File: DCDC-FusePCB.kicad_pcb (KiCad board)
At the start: 2 copper layers, 59 x 39 mm, 11 parts, among them J1 Conn_01x02_Socket, J2 Conn_01x02_Socket

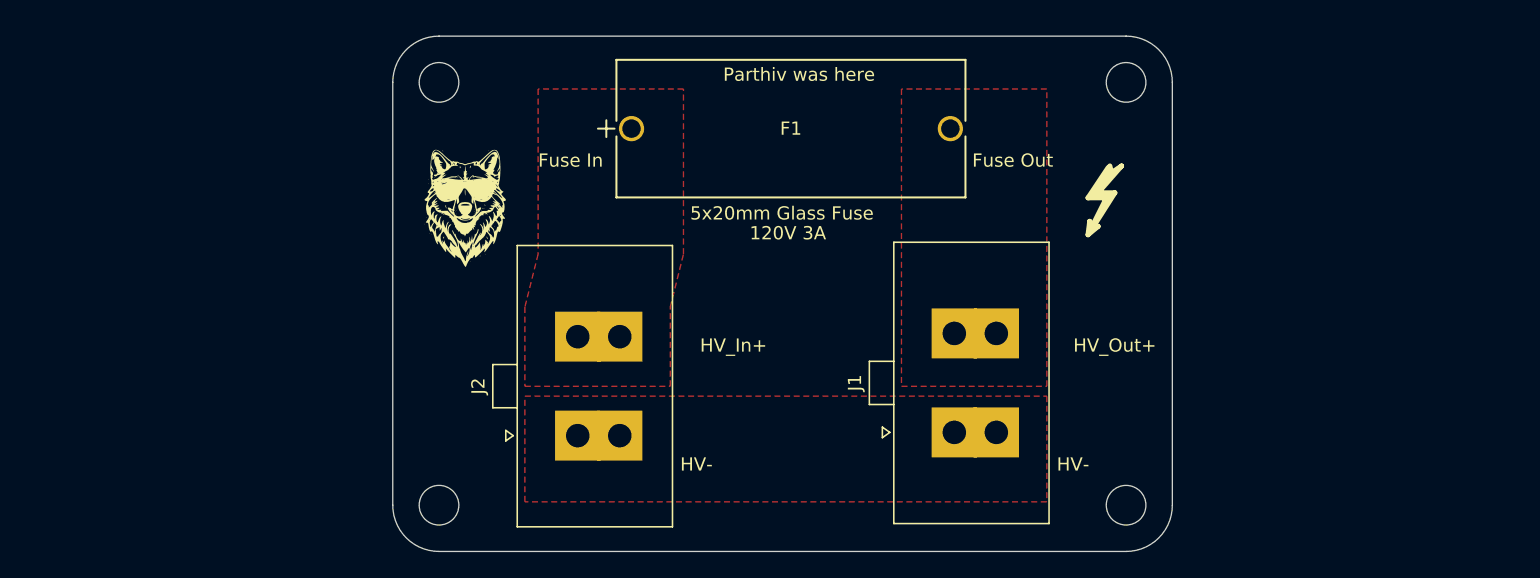
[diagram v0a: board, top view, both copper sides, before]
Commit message: precharge board
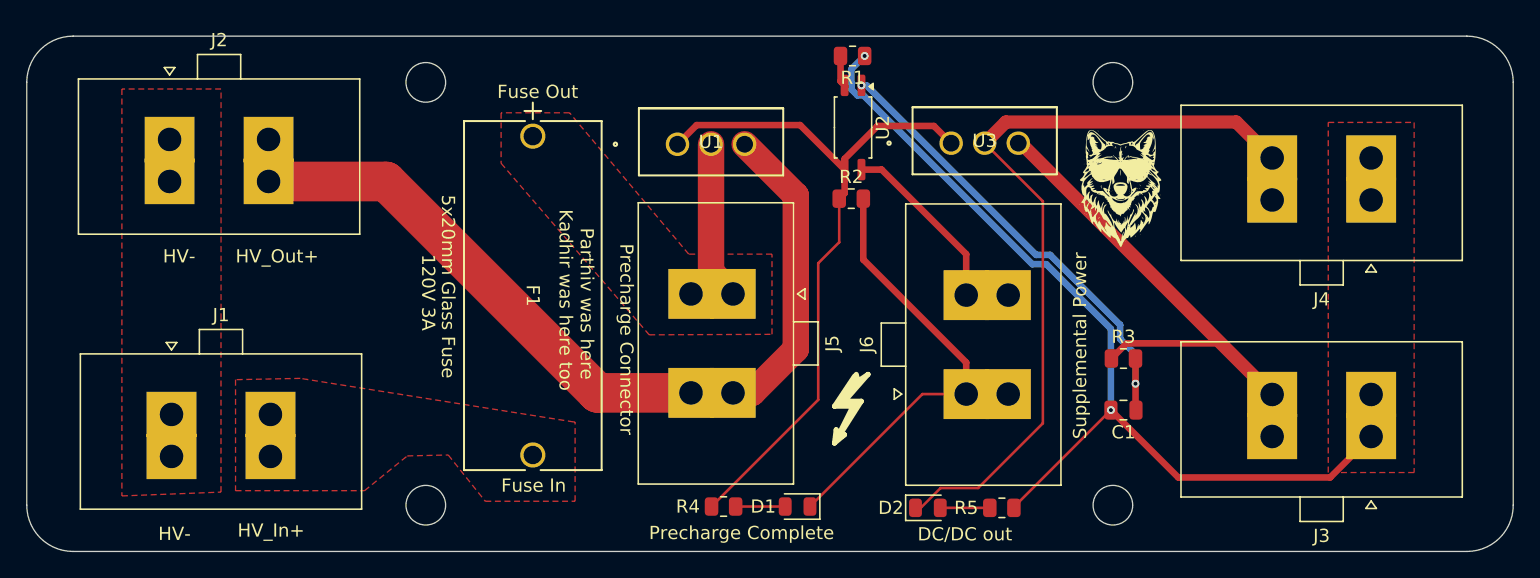
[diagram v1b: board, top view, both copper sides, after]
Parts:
- added C1: 4.7uF, Capacitor_SMD:C_0805_2012Metric, F.Cu at (164.8, 95.3)
- added D1: LED, LED_SMD:LED_0805_2012Metric, F.Cu at (140.1, 102.6)
- added D2: LED, LED_SMD:LED_0805_2012Metric, F.Cu at (150.0, 102.7)
- added J3: Conn_01x02_Socket, Connector_Molex:Molex_Sabre_43160-0102_1x02_P7.49mm_Vertical, F.Cu at (183.5, 94.1)
- added J4: Conn_01x02_Socket, Connector_Molex:Molex_Sabre_43160-0102_1x02_P7.49mm_Vertical, F.Cu at (183.5, 76.2)
- added J5: Precharge Resistor Breakout, Connector_Molex:Molex_Sabre_43160-0102_1x02_P7.49mm_Vertical, F.Cu at (132.1, 86.5)
- added J6: Conn_01x02_Socket, Connector_Molex:Molex_Sabre_43160-0102_1x02_P7.49mm_Vertical, F.Cu at (156.1, 94.1)
- added R1: 10k, Resistor_SMD:R_0805_2012Metric, F.Cu at (144.3, 68.5)
- added R2: 10k, Resistor_SMD:R_0805_2012Metric, F.Cu at (144.2, 79.3)
- added R3: 100k, Resistor_SMD:R_0805_2012Metric, F.Cu at (164.8, 91.4)
- added R4: 22.1k, Resistor_SMD:R_0805_2012Metric, F.Cu at (134.5, 102.6)
- added R5: 22.1k, Resistor_SMD:R_0805_2012Metric, F.Cu at (155.6, 102.7)
- added U1: FDP3651U, footprints:TO-220-3_16P51X10P67_ONS, F.Cu at (131.0, 75.2)
- added U2: TCMT1100, Package_SO:SOP-4_4.4x2.6mm_P1.27mm, F.Cu at (144.3, 73.9)
- added U3: FDP3651U, footprints:TO-220-3_16P51X10P67_ONS, F.Cu at (151.8, 75.1)
- moved J1 62.5 mm to (92.8, 98.8), turned to 0 degrees
- moved G*** 49.6 mm to (164.6, 78.5)
- moved J2 39.1 mm to (92.6, 78.0), turned to 0 degrees
- moved REF** 24.8 mm to (143.3, 95.8)
- moved G*** 23.4 mm to (133.1, 100.6)
- moved G*** 15.7 mm to (153.7, 96.6)
- moved F1 7.49 mm to (120.1, 74.6), turned to -90 degrees
- moved REF** 1.00 mm to (164.0, 70.5)
- moved REF** 1.00 mm to (112.0, 102.5)
- moved REF** 1.00 mm to (112.0, 70.5)
- moved REF** 1.00 mm to (164.0, 102.5)
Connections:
- net Net-(J1-Pin_1) renamed GNDin
- net Net-(J1-Pin_2) renamed HVin
- F1 pad 1: Net-(J2-Pin_2) -> Net-(J5-Pin_1)
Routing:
- net GNDout: track 0.00 -> 69.8 mm, vias 0 -> 2
- net Net-(J2-Pin_2): track 0.00 -> 61.8 mm
- net DC/DC out: track 0.00 -> 58.9 mm
- net Gate_Drive: track 0.00 -> 54.8 mm
- net LowPassIn: track 0.00 -> 41.3 mm
- net LowPassOut: track 0.00 -> 35.9 mm, vias 0 -> 2
- net GNDsupp: track 0.00 -> 33.4 mm
- net +12Vsupp: track 0.00 -> 13.7 mm
- net Net-(J5-Pin_1): track 0.00 -> 12.0 mm
- net Net-(D2-A): track 0.00 -> 3.75 mm
- net Net-(D1-A): track 0.00 -> 3.75 mm
- net Net-(R1-Pad2): track 0.00 -> 2.35 mm
- added copper zone on F.Cu, net GNDout
- added copper zone on F.Cu, net Net-(J5-Pin_1)
- removed copper zone on F.Cu, net Net-(J2-Pin_2)
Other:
- board size 59 x 39 mm -> 112.5 x 39 mm
- board text added: "DC/DC out"
- board text added: "Kadhir was here too"
- board text added: "Precharge Complete"
- board text added: "Precharge Connector"
- board text added: "Supplemental Power"
